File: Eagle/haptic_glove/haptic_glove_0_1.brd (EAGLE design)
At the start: 100 x 81.3 mm, 58 parts, among them U1 DRV2605L, U2 DRV2605L, U3 DRV2605L, U4 DRV2605L, U5 MPU-6050-1, U6 MCP73833, X1 TSW-121-07-G-S, X2 TSW-121-07-G-S, X3 TSW-121-07-G-S, X4 TSW-121-07-G-S

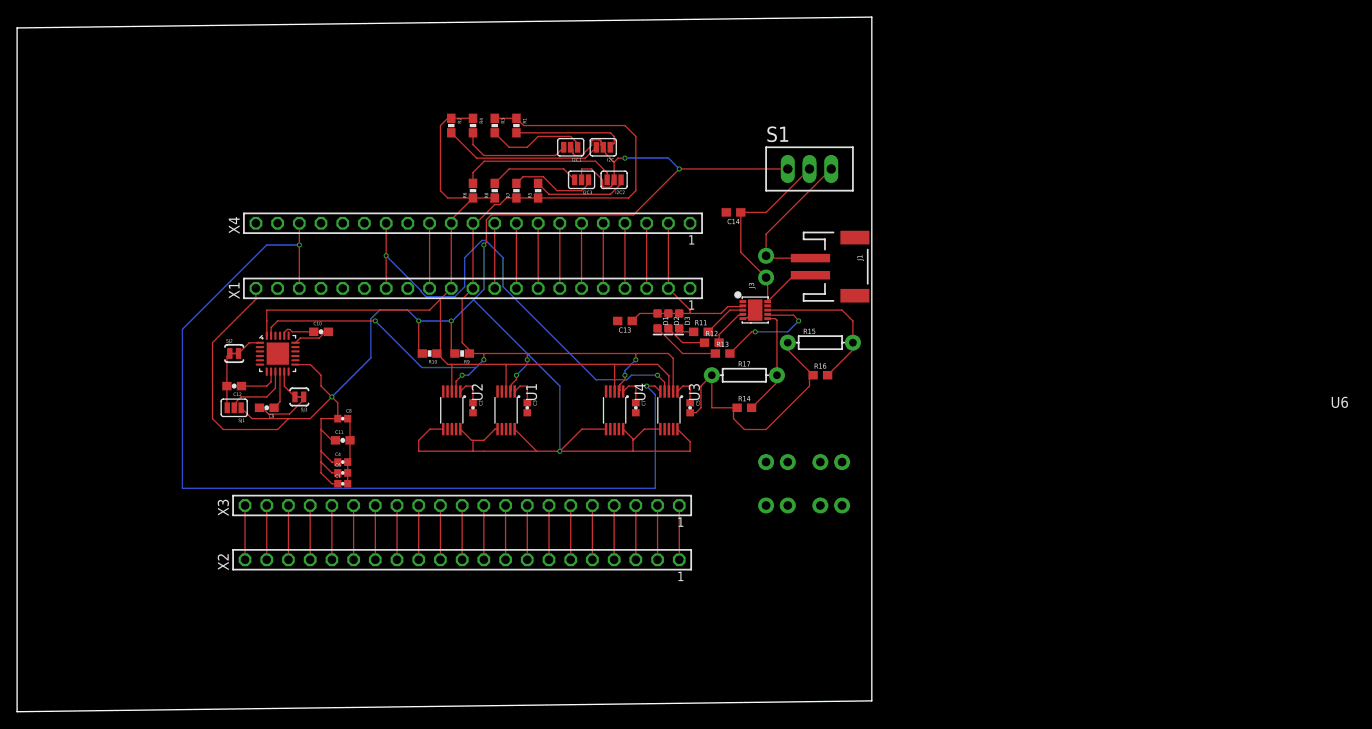
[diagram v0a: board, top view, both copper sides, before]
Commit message: Updated schematic and board design
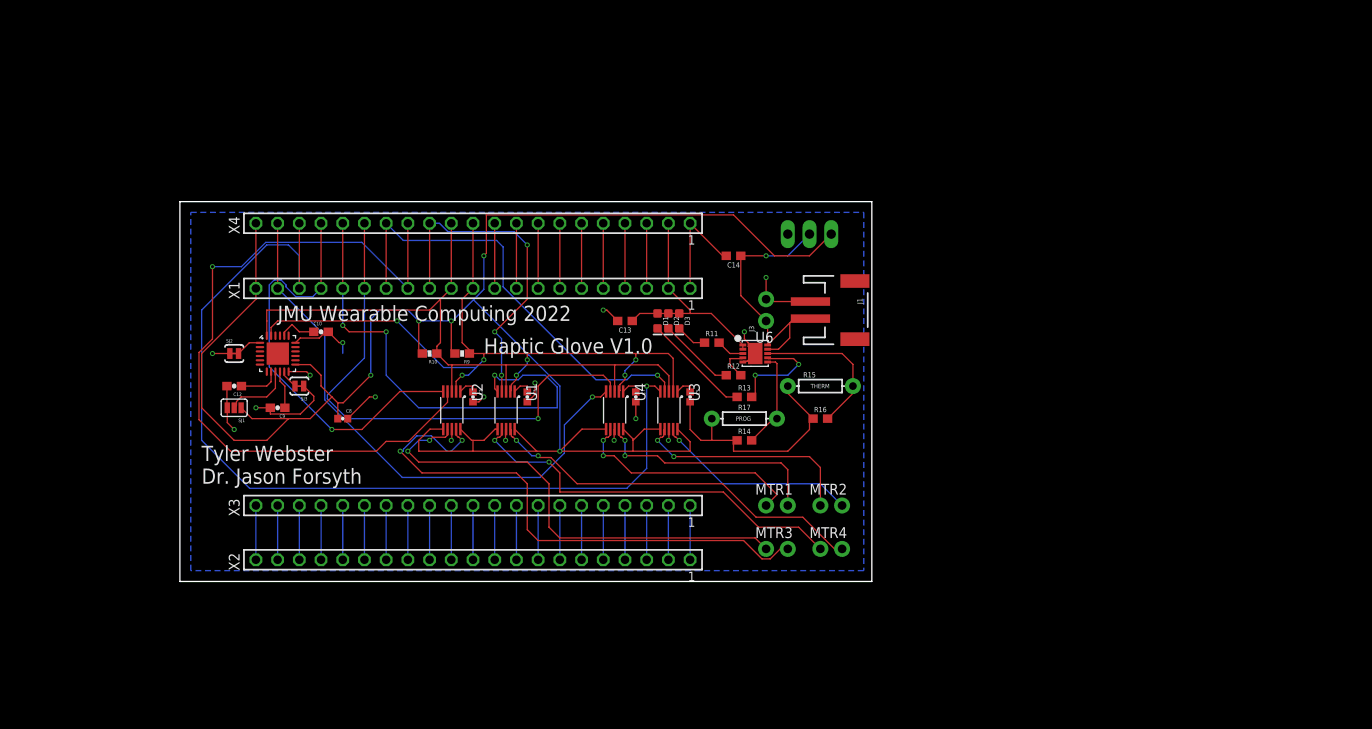
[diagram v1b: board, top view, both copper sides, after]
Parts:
- removed C1, C4, C6: 1.0uF, SparkFun-Capacitors:0402-CAP
- removed C11: 0.1uF, SparkFun:0603-CAP
- removed I2C, I2C1, I2C2, I2C3: JUMPER-PAD-3-NC_BY_PASTE, SparkFun-Passives:PAD-JUMPER-3-NC_BY_PASTE_YES_SILK_FULL_BOX
- removed JP5, JP7: (no value), SparkFun-Connectors:1X02@1
- removed R1, R2, R3, R4, R5, R6, R7, R8: 2.2k, SparkFun-Resistors:0603-RES
- added MTR3, MTR4: (no value), SparkFun-Connectors:1X02@1
- R10, R9: value 10k -> 2.2k
- moved S1 7.62 mm to (92.7, 55.9), flipped to the bottom
- moved R13 5.68 mm to (85.1, 36.8)
- moved U6 5.08 mm to (86.4, 41.9)
- moved C14 5.08 mm to (83.8, 53.3)
- moved J1 5.08 mm to (96.5, 47.0)
- moved J3 5.08 mm to (87.6, 45.7)
- moved R15 5.08 mm to (94.0, 38.1)
- moved R16 5.08 mm to (94.0, 34.3)
- moved R17 5.08 mm to (85.1, 34.3)
- moved R12 4.58 mm to (83.8, 39.4)
- moved R14 3.81 mm to (85.1, 31.8)
- moved R11 1.80 mm to (81.3, 43.2)
- moved SJ3 1.27 mm to (33.0, 38.1)
- moved X2 1.27 mm to (53.3, 17.8)
- moved X3 1.27 mm to (53.3, 24.1)
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- renumbered JP2 to MTR2, JP3 to MTR1
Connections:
- removed net INT: U5.12
- removed net N$15: I2C1.3, R4.2
- removed net N$16: I2C1.1, R3.2
- removed net N$24: I2C2.3, R6.2
- removed net N$25: I2C2.1, R5.2
- removed net N$33: I2C3.3, R8.2
- removed net N$34: I2C3.1, R7.2
- removed net N$8: I2C.3, R2.2
- removed net N$9: I2C.1, R1.2
- net GND: now also U5.12; no longer C1.2, C11.2, C4.2, C6.2
- net N$13: now also MTR3.1; no longer MTR1.1
- net N$14: now also MTR3.2; no longer MTR1.2
- net N$22: now also MTR2.1; no longer JP5.1
- net N$23: now also MTR2.2; no longer JP5.2
- net N$31: now also MTR1.1; no longer JP7.1
- net N$32: now also MTR1.2; no longer JP7.2
- net N$6: now also MTR4.1; no longer MTR2.1
- net N$7: now also MTR4.2; no longer MTR2.2
- net SCL: no longer R1.1, R3.1, R5.1, R7.1
- net SDA: no longer R2.1, R4.1, R6.1, R8.1
- net VCC: no longer C1.1, C11.1, C4.1, C6.1, I2C.2, I2C1.2, I2C2.2, I2C3.2
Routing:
- net N$11: track 0.00 -> 86.7 mm, vias 0 -> 1
- net N$30: track 0.00 -> 65.7 mm, vias 0 -> 1
- net N$13: track 0.00 -> 65.3 mm, vias 0 -> 2
- net N$29: track 0.00 -> 62.2 mm, vias 0 -> 1
- net N$5: track 0.00 -> 56.8 mm, vias 0 -> 3
- net N$14: track 0.00 -> 55.7 mm, vias 0 -> 2
- net N$12: track 0.00 -> 50.1 mm, vias 0 -> 1
- net N$7: track 0.00 -> 46.5 mm, vias 0 -> 2
- net N$6: track 0.00 -> 45.0 mm, vias 0 -> 2
- net SCL: track 132.9 -> 88.5 mm
- net N$4: track 7.62 -> 39.2 mm, vias 0 -> 3
- net N$32: track 0.00 -> 27.6 mm, vias 0 -> 2
- net VCC: track 259.2 -> 231.7 mm, vias 7 -> 5
- net N$31: track 0.00 -> 27.4 mm, vias 0 -> 2
- net N$23: track 0.00 -> 26.6 mm, vias 0 -> 2
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- added copper zone on layer 16, net GND
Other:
- board size 100 x 81.3 mm -> 81 x 44.4 mm
- board text added: "3V3"
- board text added: "Gnd"
- board text added: "Haptic Glove V1.0"
- board text added: "JMU Wearable Computing 2022"
- board text added: "MTR1"
- board text added: "MTR2"
- board text added: "MTR3"
- board text added: "MTR4"
- board text added: "PROG"
- board text added: "THERM"
- board text added: "Tyler Webster Dr. Jason Forsyth"
